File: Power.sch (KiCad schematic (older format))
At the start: 16 parts, among them J4 5V_OUT, J5 3.3V _OUT, J6 12V_OUT, U5 ACS711xLCTR-25AB, U6 D24V90F5

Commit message: Added footprints
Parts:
- BT1: footprint (none) -> Connector_AMASS:AMASS_XT60-F_1x02_P7.20mm_Vertical
- C3: footprint (none) -> Capacitor_SMD:C_0603_1608Metric_Pad1.05x0.95mm_HandSolder
- C4, C5, C6, C7: footprint (none) -> Capacitor_THT:CP_Radial_D10.0mm_P5.00mm
- F4, F5: footprint (none) -> Fuse:Fuse_0805_2012Metric_Pad1.15x1.40mm_HandSolder
- J4, J5, J6: footprint (none) -> TerminalBlock_TE-Connectivity:TerminalBlock_TE_282834-2_1x02_P2.54mm_Horizontal
- R19, R20, R21: footprint (none) -> Resistor_SMD:R_0603_1608Metric_Pad1.05x0.95mm_HandSolder
- U6: footprint (none) -> TurtlebotController:Pololu_D24V90F5
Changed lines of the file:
@@
 F 0 "BT1" H 1258 2346 50  0000 L CNN
 F 1 "Battery" H 1258 2255 50  0000 L CNN
-F 2 "" V 1150 2360 50  0001 C CNN
+F 2 "Connector_AMASS:AMASS_XT60-F_1x02_P7.20mm_Vertical" V 1150 2360 50  0001 C CNN
 F 3 "~" V 1150 2360 50  0001 C CNN
 	1    1150 2300
@@
 F 0 "F4" V 1403 2100 50  0000 C CNN
 F 1 "Fuse" V 1494 2100 50  0000 C CNN
-F 2 "" V 1530 2100 50  0001 C CNN
+F 2 "Fuse:Fuse_0805_2012Metric_Pad1.15x1.40mm_HandSolder" V 1530 2100 50  0001 C CNN
 F 3 "~" H 1600 2100 50  0001 C CNN
 	1    1600 2100
@@
 F 0 "C3" H 1642 1596 50  0000 L CNN
 F 1 "0.1uF" H 1642 1505 50  0000 L CNN
-F 2 "" H 1550 1550 50  0001 C CNN
+F 2 "Capacitor_SMD:C_0603_1608Metric_Pad1.05x0.95mm_HandSolder" H 1550 1550 50  0001 C CNN
 F 3 "~" H 1550 1550 50  0001 C CNN
 	1    1550 1550
@@
 F 0 "R19" V 2254 1250 50  0000 C CNN
 F 1 "10K" V 2345 1250 50  0000 C CNN
-F 2 "" H 2450 1250 50  0001 C CNN
+F 2 "Resistor_SMD:R_0603_1608Metric_Pad1.05x0.95mm_HandSolder" H 2450 1250 50  0001 C CNN
 F 3 "~" H 2450 1250 50  0001 C CNN
 	1    2450 1250
@@
 F 0 "C4" V 4455 1300 50  0000 C CNN
 F 1 "1000uF" V 4364 1300 50  0000 C CNN
-F 2 "" H 4238 1150 50  0001 C CNN
+F 2 "Capacitor_THT:CP_Radial_D10.0mm_P5.00mm" H 4238 1150 50  0001 C CNN
 F 3 "~" H 4200 1300 50  0001 C CNN
 	1    4200 1300
@@
 F 0 "C5" V 4455 1700 50  0000 C CNN
 F 1 "1000uF" V 4364 1700 50  0000 C CNN
-F 2 "" H 4238 1550 50  0001 C CNN
+F 2 "Capacitor_THT:CP_Radial_D10.0mm_P5.00mm" H 4238 1550 50  0001 C CNN
 F 3 "~" H 4200 1700 50  0001 C CNN
 	1    4200 1700
@@
 F 0 "C6" V 4455 2150 50  0000 C CNN
 F 1 "1000uF" V 4364 2150 50  0000 C CNN
-F 2 "" H 4238 2000 50  0001 C CNN
+F 2 "Capacitor_THT:CP_Radial_D10.0mm_P5.00mm" H 4238 2000 50  0001 C CNN
 F 3 "~" H 4200 2150 50  0001 C CNN
 	1    4200 2150
@@
 F 0 "C7" V 4455 2550 50  0000 C CNN
 F 1 "1000uF" V 4364 2550 50  0000 C CNN
-F 2 "" H 4238 2400 50  0001 C CNN
+F 2 "Capacitor_THT:CP_Radial_D10.0mm_P5.00mm" H 4238 2400 50  0001 C CNN
 F 3 "~" H 4200 2550 50  0001 C CNN
 	1    4200 2550
@@
 F 0 "U6" H 8900 2625 50  0000 C CNN
 F 1 "D24V90F5" H 8900 2534 50  0000 C CNN
-F 2 "" H 8900 1850 50  0001 C CNN
+F 2 "TurtlebotController:Pololu_D24V90F5" H 8900 1850 50  0001 C CNN
 F 3 "" H 8900 1850 50  0001 C CNN
 	1    8900 1850
@@
 F 0 "J4" V 1272 4230 50  0000 L CNN
 F 1 "5V_OUT" V 1363 4230 50  0000 L CNN
-F 2 "" H 1400 4150 50  0001 C CNN
+F 2 "TerminalBlock_TE-Connectivity:TerminalBlock_TE_282834-2_1x02_P2.54mm_Horizontal" H 1400 4150 50  0001 C CNN
 F 3 "~" H 1400 4150 50  0001 C CNN
 	1    1400 4150
@@
 F 0 "J5" V 1922 4230 50  0000 L CNN
 F 1 "3.3V _OUT" V 2013 4230 50  0000 L CNN
-F 2 "" H 2050 4150 50  0001 C CNN
+F 2 "TerminalBlock_TE-Connectivity:TerminalBlock_TE_282834-2_1x02_P2.54mm_Horizontal" H 2050 4150 50  0001 C CNN
 F 3 "~" H 2050 4150 50  0001 C CNN
 	1    2050 4150
@@
 F 0 "J6" V 2572 4230 50  0000 L CNN
 F 1 "12V_OUT" V 2663 4230 50  0000 L CNN
-F 2 "" H 2700 4150 50  0001 C CNN
+F 2 "TerminalBlock_TE-Connectivity:TerminalBlock_TE_282834-2_1x02_P2.54mm_Horizontal" H 2700 4150 50  0001 C CNN
 F 3 "~" H 2700 4150 50  0001 C CNN
 	1    2700 4150
@@
 F 0 "R20" H 5959 1496 50  0000 L CNN
 F 1 "270 Ohm" H 5959 1405 50  0000 L CNN
-F 2 "" H 5900 1450 50  0001 C CNN
+F 2 "Resistor_SMD:R_0603_1608Metric_Pad1.05x0.95mm_HandSolder" H 5900 1450 50  0001 C CNN
 F 3 "~" H 5900 1450 50  0001 C CNN
 	1    5900 1450
@@
 F 0 "R21" H 5959 1796 50  0000 L CNN
 F 1 "70 Ohm" H 5959 1705 50  0000 L CNN
-F 2 "" H 5900 1750 50  0001 C CNN
+F 2 "Resistor_SMD:R_0603_1608Metric_Pad1.05x0.95mm_HandSolder" H 5900 1750 50  0001 C CNN
 F 3 "~" H 5900 1750 50  0001 C CNN
 	1    5900 1750
@@
 F 0 "F5" V 7797 1550 50  0000 C CNN
 F 1 "Fuse" V 7706 1550 50  0000 C CNN
-F 2 "" V 7530 1550 50  0001 C CNN
+F 2 "Fuse:Fuse_0805_2012Metric_Pad1.15x1.40mm_HandSolder" V 7530 1550 50  0001 C CNN
 F 3 "~" H 7600 1550 50  0001 C CNN
 	1    7600 1550

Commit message: Added BOM
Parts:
- BT1: DigiKey (none) -> 1568-1816-ND
- C4, C5, C6, C7: DigiKey (none) -> 493-12561-1-ND
- J4, J5, J6: DigiKey (none) -> A98333-ND
- R19: DigiKey (none) -> 311-10KGRCT-ND
- R20: DigiKey (none) -> RR08P270DCT-ND
- R21: DigiKey (none) -> 311-75.0HRCT-ND
- U5: DigiKey (none) -> 620-1373-1-ND
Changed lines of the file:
@@
 F 2 "Connector_AMASS:AMASS_XT60-F_1x02_P7.20mm_Vertical" V 1150 2360 50  0001 C CNN
 F 3 "~" V 1150 2360 50  0001 C CNN
+F 4 " 1568-1816-ND " H 1150 2300 50  0001 C CNN "DigiKey"
 	1    1150 2300
 	1    0    0    -1
@@
 F 2 "Package_SO:SOIC-8_3.9x4.9mm_P1.27mm" H 2600 1650 50  0001 L CIN
 F 3 "http://www.allegromicro.com/~/Media/Files/Datasheets/ACS711-Datasheet.ashx" H 2250 1700 50  0001 C CNN
+F 4 " 620-1373-1-ND" H 2250 1700 50  0001 C CNN "DigiKey"
 	1    2250 1700
 	0    -1   -1   0
@@
 F 2 "Resistor_SMD:R_0603_1608Metric_Pad1.05x0.95mm_HandSolder" H 2450 1250 50  0001 C CNN
 F 3 "~" H 2450 1250 50  0001 C CNN
+F 4 " 311-10KGRCT-ND " H 2450 1250 50  0001 C CNN "DigiKey"
 	1    2450 1250
 	0    1    1    0
@@
 F 2 "Capacitor_THT:CP_Radial_D10.0mm_P5.00mm" H 4238 1150 50  0001 C CNN
 F 3 "~" H 4200 1300 50  0001 C CNN
+F 4 "493-12561-1-ND" H 4200 1300 50  0001 C CNN "DigiKey"
 	1    4200 1300
 	0    -1   -1   0
@@
 F 2 "Capacitor_THT:CP_Radial_D10.0mm_P5.00mm" H 4238 1550 50  0001 C CNN
 F 3 "~" H 4200 1700 50  0001 C CNN
+F 4 "493-12561-1-ND" H 4200 1700 50  0001 C CNN "DigiKey"
 	1    4200 1700
 	0    -1   -1   0
@@
 F 2 "Capacitor_THT:CP_Radial_D10.0mm_P5.00mm" H 4238 2000 50  0001 C CNN
 F 3 "~" H 4200 2150 50  0001 C CNN
+F 4 "493-12561-1-ND" H 4200 2150 50  0001 C CNN "DigiKey"
 	1    4200 2150
 	0    -1   -1   0
@@
 F 2 "Capacitor_THT:CP_Radial_D10.0mm_P5.00mm" H 4238 2400 50  0001 C CNN
 F 3 "~" H 4200 2550 50  0001 C CNN
+F 4 "493-12561-1-ND" H 4200 2550 50  0001 C CNN "DigiKey"
 	1    4200 2550
 	0    -1   -1   0
@@
 F 2 "TerminalBlock_TE-Connectivity:TerminalBlock_TE_282834-2_1x02_P2.54mm_Horizontal" H 1400 4150 50  0001 C CNN
 F 3 "~" H 1400 4150 50  0001 C CNN
+F 4 "A98333-ND" H 1400 4150 50  0001 C CNN "DigiKey"
 	1    1400 4150
 	0    1    1    0
@@
 F 2 "TerminalBlock_TE-Connectivity:TerminalBlock_TE_282834-2_1x02_P2.54mm_Horizontal" H 2050 4150 50  0001 C CNN
 F 3 "~" H 2050 4150 50  0001 C CNN
+F 4 "A98333-ND" H 2050 4150 50  0001 C CNN "DigiKey"
 	1    2050 4150
 	0    1    1    0
@@
 F 2 "TerminalBlock_TE-Connectivity:TerminalBlock_TE_282834-2_1x02_P2.54mm_Horizontal" H 2700 4150 50  0001 C CNN
 F 3 "~" H 2700 4150 50  0001 C CNN
+F 4 "A98333-ND" H 2700 4150 50  0001 C CNN "DigiKey"
 	1    2700 4150
 	0    1    1    0
@@
 F 2 "Resistor_SMD:R_0603_1608Metric_Pad1.05x0.95mm_HandSolder" H 5900 1450 50  0001 C CNN
 F 3 "~" H 5900 1450 50  0001 C CNN
+F 4 " RR08P270DCT-ND " H 5900 1450 50  0001 C CNN "DigiKey"
 	1    5900 1450
 	1    0    0    -1
@@
 F 2 "Resistor_SMD:R_0603_1608Metric_Pad1.05x0.95mm_HandSolder" H 5900 1750 50  0001 C CNN
 F 3 "~" H 5900 1750 50  0001 C CNN
+F 4 " 311-75.0HRCT-ND " H 5900 1750 50  0001 C CNN "DigiKey"
 	1    5900 1750
 	1    0    0    -1

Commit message: Some fixes
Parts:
- U5: DigiKey 620-1373-1-ND -> 620-1372-1-ND
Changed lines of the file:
@@
 F 2 "Package_SO:SOIC-8_3.9x4.9mm_P1.27mm" H 2600 1650 50  0001 L CIN
 F 3 "http://www.allegromicro.com/~/Media/Files/Datasheets/ACS711-Datasheet.ashx" H 2250 1700 50  0001 C CNN
-F 4 " 620-1373-1-ND" H 2250 1700 50  0001 C CNN "DigiKey"
+F 4 " 620-1372-1-ND" H 2250 1700 50  0001 C CNN "DigiKey"
 	1    2250 1700
 	0    -1   -1   0

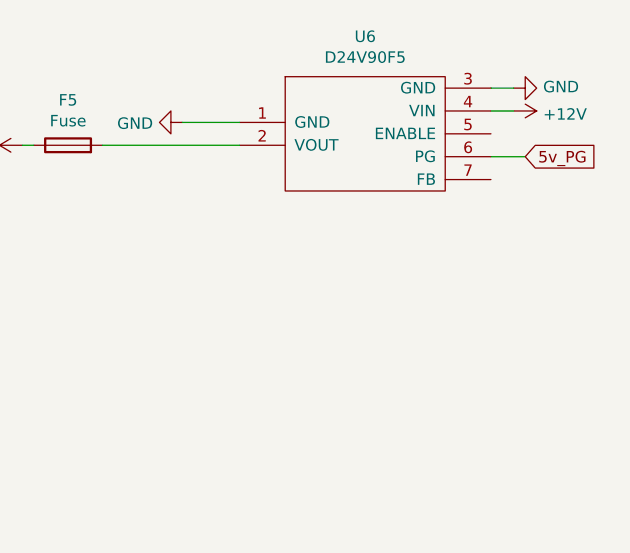
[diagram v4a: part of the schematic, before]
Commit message: Rev B
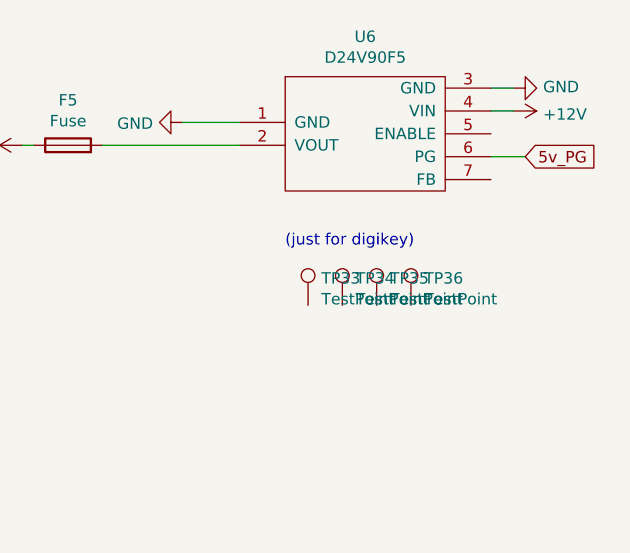
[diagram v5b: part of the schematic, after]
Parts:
- added TP33, TP34, TP35, TP36: TestPoint, symbol Connector:TestPoint
- C3: DigiKey (none) -> 399-1100-1-ND
- R20: DigiKey RR08P270DCT-ND -> RR08P270DCT-ND
- R21: DigiKey 311-75.0HRCT-ND -> 311-75.0HRCT-ND
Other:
- note added: "(just for digikey)"
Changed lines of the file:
@@
 F 2 "Capacitor_SMD:C_0603_1608Metric_Pad1.05x0.95mm_HandSolder" H 1550 1550 50  0001 C CNN
 F 3 "~" H 1550 1550 50  0001 C CNN
+F 4 "399-1100-1-ND" H 1550 1550 50  0001 C CNN "DigiKey"
 	1    1550 1550
 	1    0    0    -1
@@
 F 2 "Resistor_SMD:R_0603_1608Metric_Pad1.05x0.95mm_HandSolder" H 5900 1450 50  0001 C CNN
 F 3 "~" H 5900 1450 50  0001 C CNN
-F 4 " RR08P270DCT-ND " H 5900 1450 50  0001 C CNN "DigiKey"
+F 4 "RR08P270DCT-ND " H 5900 1450 50  0001 C CNN "DigiKey"
 	1    5900 1450
 	1    0    0    -1
@@
 F 2 "Resistor_SMD:R_0603_1608Metric_Pad1.05x0.95mm_HandSolder" H 5900 1750 50  0001 C CNN
 F 3 "~" H 5900 1750 50  0001 C CNN
-F 4 " 311-75.0HRCT-ND " H 5900 1750 50  0001 C CNN "DigiKey"
+F 4 "311-75.0HRCT-ND " H 5900 1750 50  0001 C CNN "DigiKey"
 	1    5900 1750
 	1    0    0    -1
@@
 Wire Wire Line
 	7750 1550 8350 1550
+Text Notes 8550 2000 0    50   ~ 0
+(just for digikey)
+$Comp
+L Connector:TestPoint TP33
+U 1 1 5EF2768A
+P 8650 2250
+F 0 "TP33" H 8708 2368 50  0000 L CNN
+F 1 "TestPoint" H 8708 2277 50  0000 L CNN
+F 2 "" H 8850 2250 50  0001 C CNN
+F 3 "~" H 8850 2250 50  0001 C CNN
+F 4 "S7037-ND" H 8650 2250 50  0001 C CNN "DigiKey"
+	1    8650 2250
+	1    0    0    -1
+$EndComp
+$Comp
+L Connector:TestPoint TP34
+U 1 1 5EF27A16
+P 8800 2250
+F 0 "TP34" H 8858 2368 50  0000 L CNN
+F 1 "TestPoint" H 8858 2277 50  0000 L CNN
+F 2 "" H 9000 2250 50  0001 C CNN
+F 3 "~" H 9000 2250 50  0001 C CNN
+F 4 "S7037-ND" H 8800 2250 50  0001 C CNN "DigiKey"
+	1    8800 2250
+	1    0    0    -1
+$EndComp
+$Comp
+L Connector:TestPoint TP35
+U 1 1 5EF27BD5
+P 8950 2250
+F 0 "TP35" H 9008 2368 50  0000 L CNN
+F 1 "TestPoint" H 9008 2277 50  0000 L CNN
+F 2 "" H 9150 2250 50  0001 C CNN
+F 3 "~" H 9150 2250 50  0001 C CNN
+F 4 "S7037-ND" H 8950 2250 50  0001 C CNN "DigiKey"
+	1    8950 2250
+	1    0    0    -1
+$EndComp
+$Comp
+L Connector:TestPoint TP36
+U 1 1 5EF27FBA
+P 9100 2250
+F 0 "TP36" H 9158 2368 50  0000 L CNN
+F 1 "TestPoint" H 9158 2277 50  0000 L CNN
+F 2 "" H 9300 2250 50  0001 C CNN
+F 3 "~" H 9300 2250 50  0001 C CNN
+F 4 "S7037-ND" H 9100 2250 50  0001 C CNN "DigiKey"
+	1    9100 2250
+	1    0    0    -1
+$EndComp
 $EndSCHEMATC
